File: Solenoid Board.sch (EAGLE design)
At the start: 0 parts

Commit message: Added frame and stm block
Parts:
- added C1, C3: 2.2 µF, rcl:C-USC0805
- added C13, C14: 4.7uF, SparkFun-Capacitors:4.7UF0603
- added C15, C16, C19: 100nF, SparkFun-Capacitors:4.7UF0603
- added C17: 0.01uf, SparkFun-Capacitors:4.7UF0603
- added C18: 1uF, SparkFun-Capacitors:4.7UF0603
- added C2: 4.7 µF, rcl:C-USC0805
- added C20, C21: 18pF, SparkFun-Capacitors:4.7UF0603
- added CF: 220 pF, rcl:C-USC0805
- added JP1, JP2, JP3, JP4, JP5, JP6, JP7, JP8: (no value), pinhead:PINHD-1X2
- added R1, R2: 13.3k, rcl:R-US_R0603
- added R10, R8: 0, SparkFun-Resistors:1KOHM-0603-1/10W-1%
- added R3: 51k, rcl:R-US_R0603
- added R4: 10k, rcl:R-US_R0603
- added R9: 47k, SparkFun-Resistors:1KOHM-0603-1/10W-1%
- added RESET1: SWITCH, DiscreteComponents:SWITCH
- added SV2: (no value), con-lsta:FE05-1
- added U$1: SHIFT_REGISTER, Solenoid_parts:SHIFT_REGISTER
- added U$2: LM27313, Solenoid_parts:LM27313
- added U$3: MBR0520LT1G, Solenoid_parts:MBR0520LT1G
- added U$4: DR73-100-R, Solenoid_parts:DR73-100-R
- added U$5: T2I, BackplaneParts:T2I
- added U$6: BOARDPNE, board_outlines:BOARDPNE
- added U$8: STM32F042K6T6, PI_Shield_Library:STM32F042K6T6
- added Y2: ECS-80-S-4X, ECS-80-S-4X:ECS-80-S-4X
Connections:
- new net +12V: R3.1, U$2.SHDN, U$5.2
- new net +24V: C2.1, CF.2, JP1.2, JP2.2, JP3.2, JP4.2, JP5.2, JP6.2, JP7.2, JP8.2, R1.1, U$3.C
- new net +3V3: C13.1, C14.1, C15.1, C16.1, C17.1, C18.1, R9.2, SV2.5, U$8.VDD, U$8.VDDA, U$8.VDDIO2
- new net +5V: C3.1, R4.1, U$1.VCC
- new net CAN_H: U$5.3
- new net CAN_L: U$5.4
- new net G: U$8.PA9
- new net GND: C1.2, C13.2, C14.2, C15.2, C16.2, C17.2, C18.2, C19.2, C20.2, C21.2, C3.2, R2.2, RESET1.P$1, SV2.1, U$1.GND, U$2.GND, U$5.1, U$8.PB8-BOOT0, U$8.VSS, U$8.VSS1
- new net N$1: JP1.1, U$1.DRAIN0
- new net N$10: C1.1, R3.2, U$2.VIN, U$4.1
- new net N$11: CF.1, R1.2, R2.1, U$2.FB
- new net N$12: U$2.SW, U$3.A, U$4.2
- new net N$15: C21.1, R8.1, Y2.2
- new net N$16: C20.1, R10.1, Y2.1
- new net N$2: JP2.1, U$1.DRAIN1
- new net N$3: JP3.1, U$1.DRAIN2
- new net N$4: JP4.1, U$1.DRAIN3
- new net N$5: JP5.1, U$1.DRAIN4
- new net N$6: JP6.1, U$1.DRAIN5
- new net N$7: JP7.1, U$1.DRAIN6
- new net N$8: JP8.1, U$1.DRAIN7
- new net N$9: R4.2, U$1.CLR
- new net NRST: C19.1, R9.1, RESET1.P$2, SV2.2, U$8.NRST
- new net OSC_IN: R10.2, U$8.PF0-OSC_IN
- new net OSC_OUT: R8.2, U$8.PF1-OSC_OUT
- new net RCK: U$8.PA15
- new net SER_IN: U$8.PA8
- new net SRCK: U$8.PA10
- new net SWCLK: SV2.3, U$8.PA14
- new net SWDIO: SV2.4, U$8.PA13
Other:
- note added: "Pin 1 (VDD)"
- note added: "Pin 17 (VDDIO2)"
- note added: "Pin 5 (VDDA)"

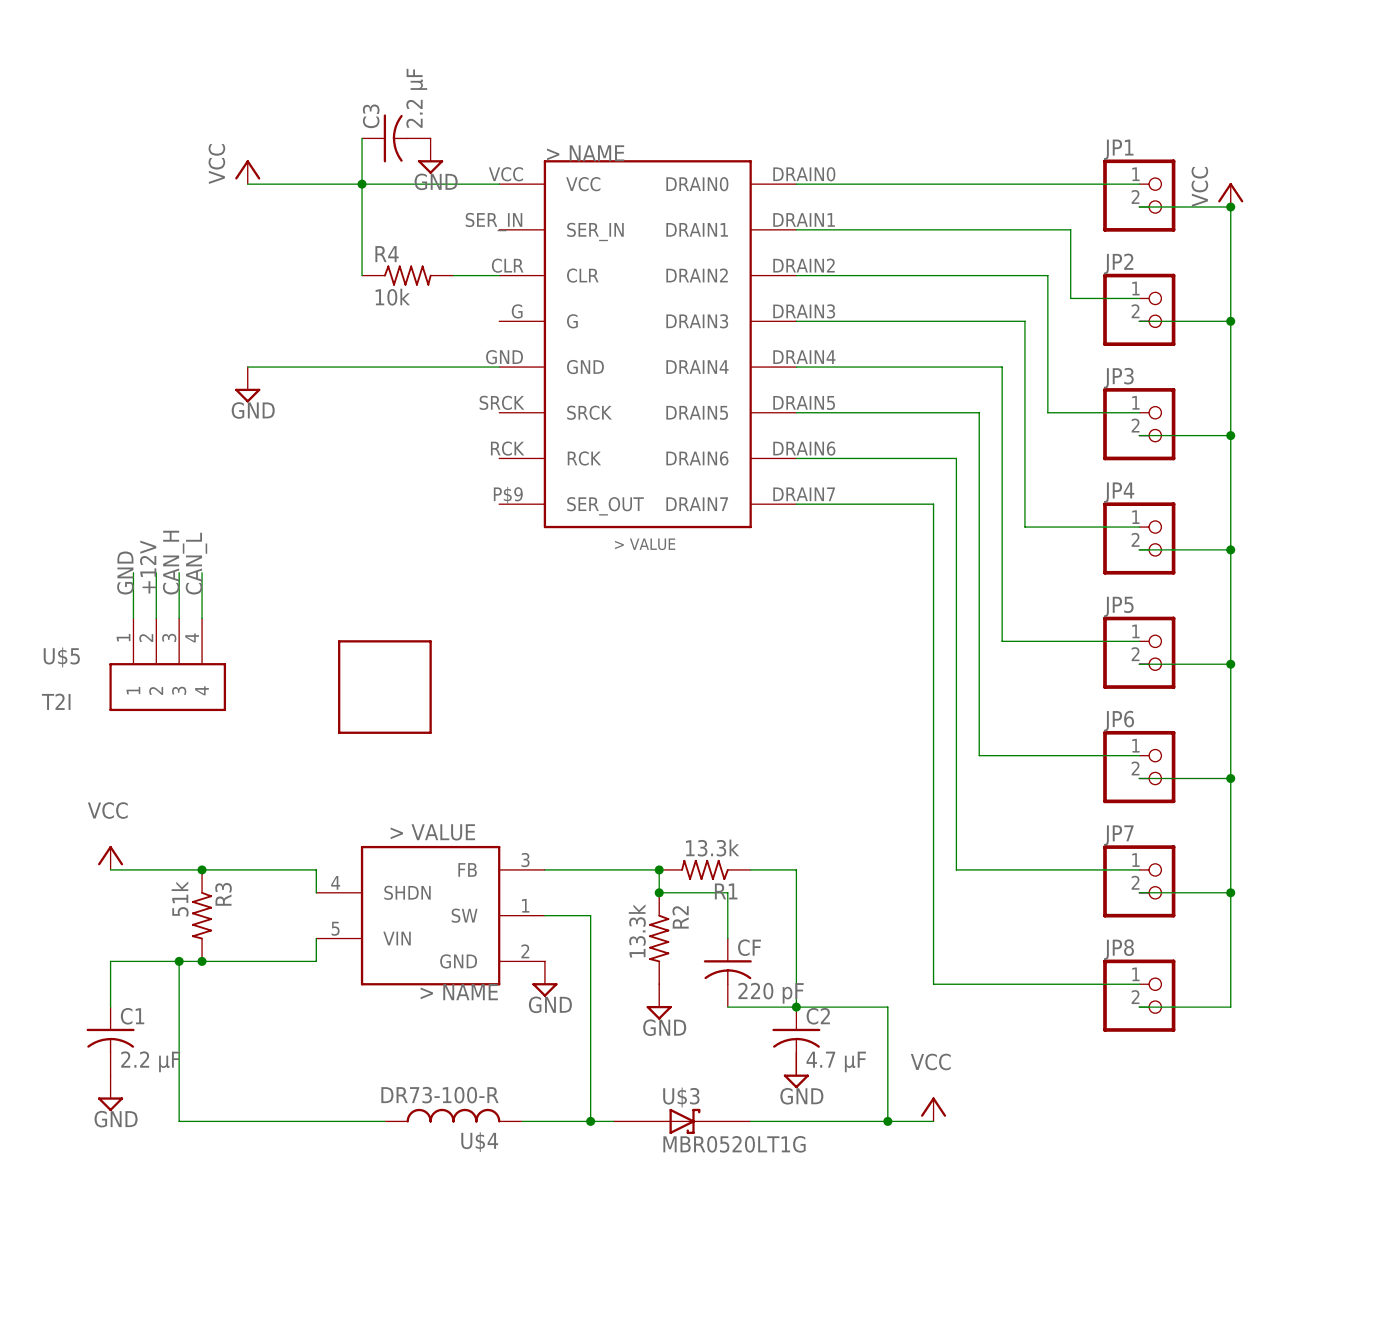
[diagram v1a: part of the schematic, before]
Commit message: Created the board layout
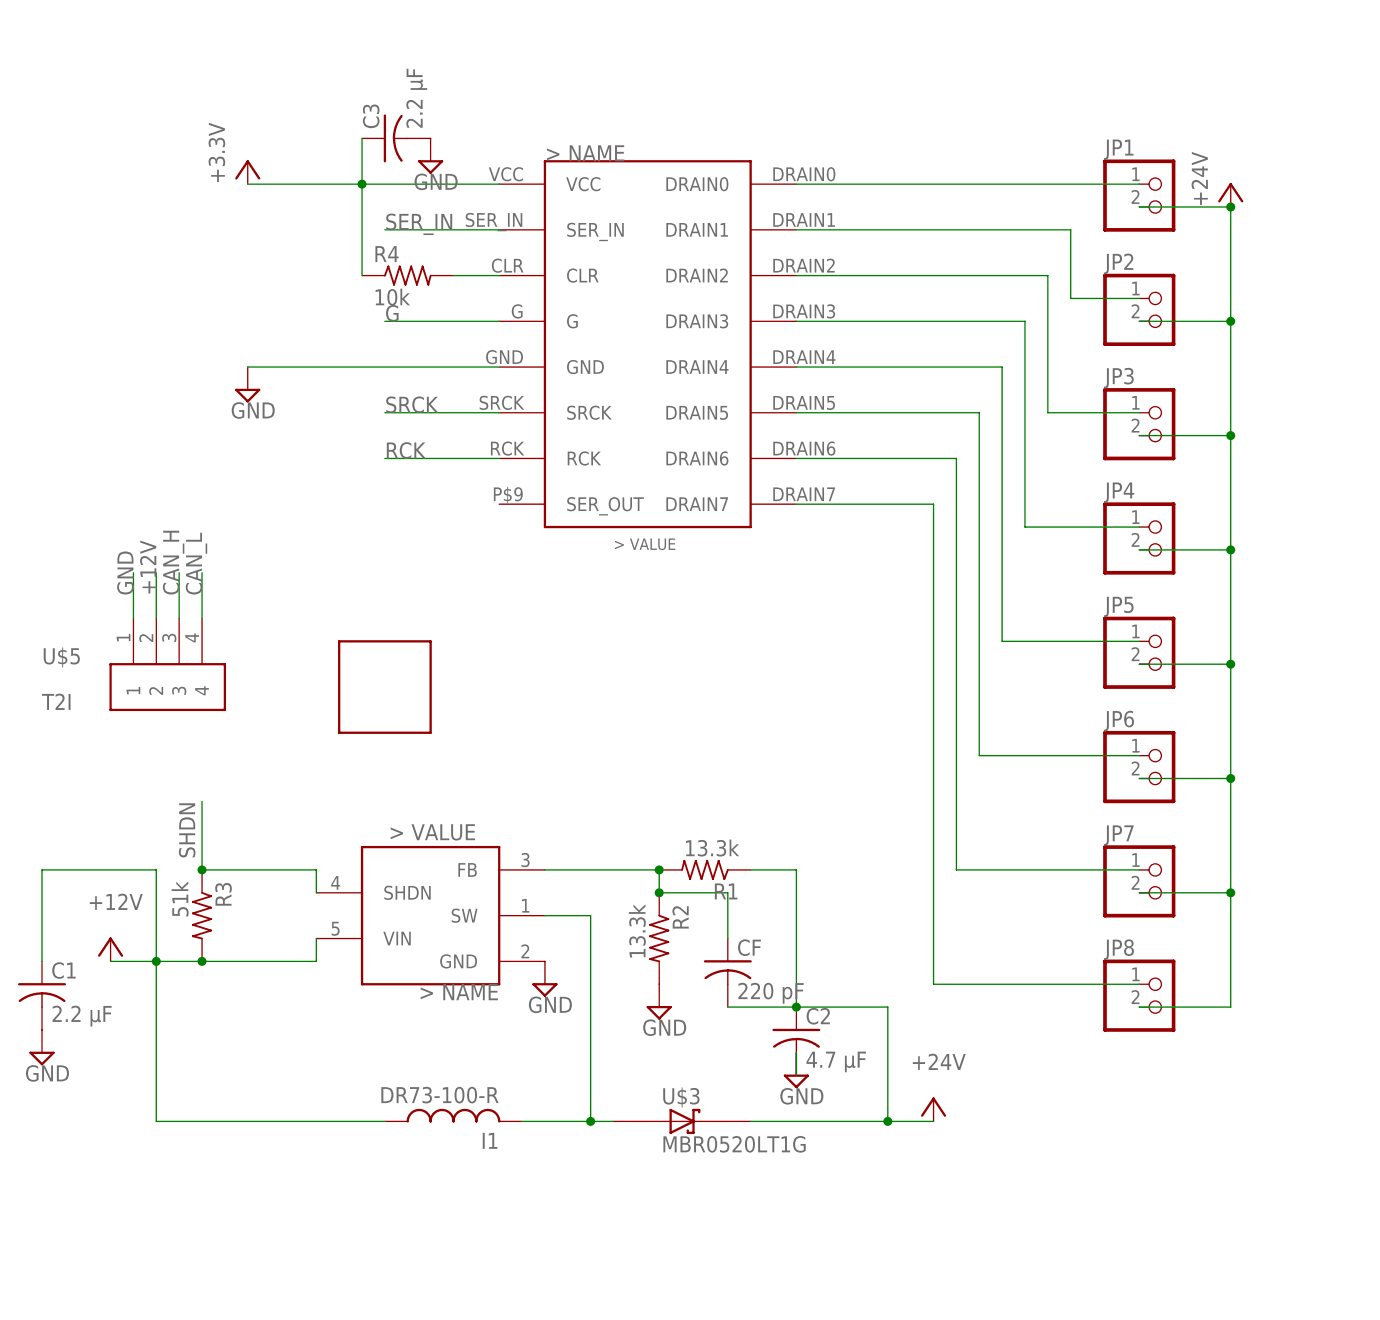
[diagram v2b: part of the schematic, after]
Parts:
- renumbered U$4 to I1
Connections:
- net +5V renamed +3.3V
- net N$1 renamed DRAIN0
- net N$11 renamed FB
- net N$12 renamed SW
- net N$2 renamed DRAIN1
- net N$3 renamed DRAIN2
- net N$4 renamed DRAIN3
- net N$5 renamed DRAIN4
- net N$6 renamed DRAIN5
- net N$7 renamed DRAIN6
- net N$8 renamed DRAIN7
- net N$9 renamed CLR
- removed net N$10: C1.1, I1.1, R3.2, U$2.VIN
- new net SHDN: R3.1, U$2.SHDN
- net +12V: now also C1.1, I1.1, R3.2, U$2.VIN; no longer R3.1, U$2.SHDN
- net G: now also U$1.G
- net GND: now also C2.2
- net RCK: now also U$1.RCK
- net SER_IN: now also U$1.SER_IN
- net SRCK: now also U$1.SRCK
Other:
- moved on the sheet: C1
